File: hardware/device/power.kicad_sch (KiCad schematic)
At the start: 46 parts, among them IC3 SP3401-02UTG, J1 POT_CONN, J2 USB, U20 TPS62A02DRL, U21 TPS560200, U22 BQ24072RGT, U23 BQ21040DBV, U26 BQ25040, U31 FUSB302B01MPX, U32 LTC2942

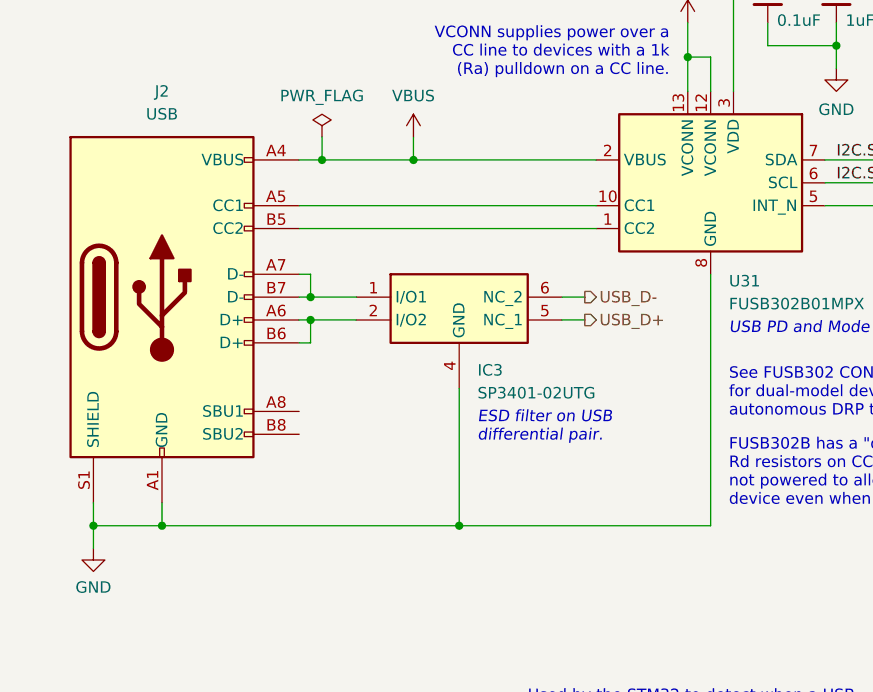
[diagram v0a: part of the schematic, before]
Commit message: feat: audio system routing
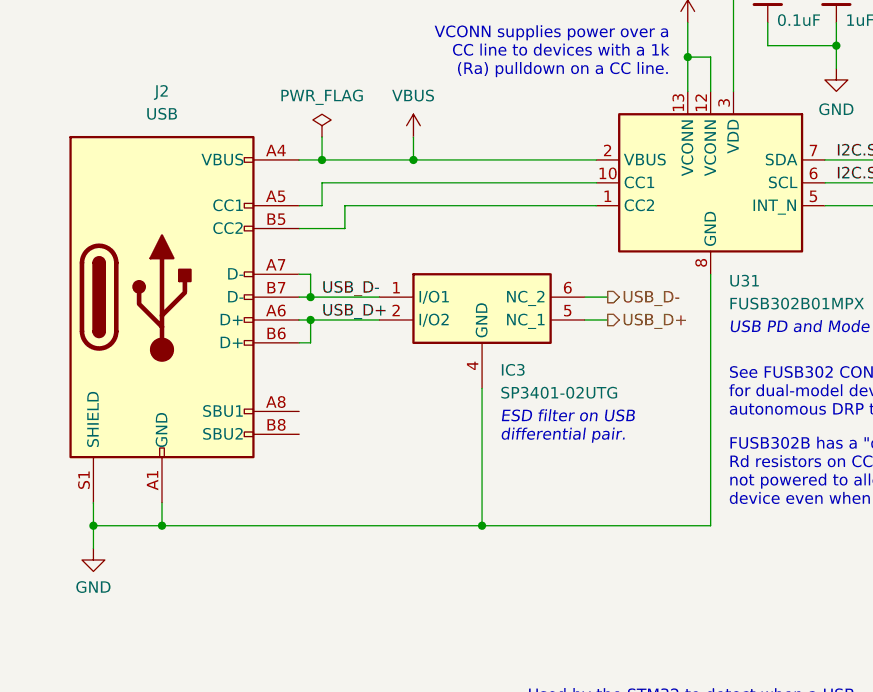
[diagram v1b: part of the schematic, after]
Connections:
- net USB_D+: now also IC3.2 (I/O2), J2.A6 (D+), J2.B6 (D+)
- net USB_D-: now also IC3.1 (I/O1), J2.A7 (D-), J2.B7 (D-)
- net at J2.B5 (CC2), U31.1 (CC2): now also U31.14 (CC2)
- net at J2.A5 (CC1), U31.10 (CC1): now also U31.11 (CC1); no longer U31.14 (CC2)
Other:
- moved on the sheet: IC3
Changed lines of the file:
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@@
 	(text "ESD filter on USB\ndifferential pair."
 		(exclude_from_sim no)
-		(at 64.262 76.2 0)
+		(at 66.802 76.2 0)
 		(effects
 			(font
@@
 	)
 	(junction
-		(at 62.23 88.9)
-		(diameter 0)
-		(color 0 0 0 0)
-	)
-	(junction
 		(at 76.2 153.67)
 		(diameter 0)
@@
 	)
 	(junction
+		(at 64.77 88.9)
+		(diameter 0)
+		(color 0 0 0 0)
+	)
+	(junction
 		(at 57.15 48.26)
 		(diameter 0)
@@
 	(wire
 		(pts
-			(xy 62.23 73.66) (xy 62.23 88.9)
+			(xy 64.77 73.66) (xy 64.77 88.9)
 		)
 		(stroke
@@
 	(wire
 		(pts
-			(xy 29.21 88.9) (xy 62.23 88.9)
+			(xy 29.21 88.9) (xy 64.77 88.9)
 		)
 		(stroke
@@
 		)
 	)
+	(wire
+		(pts
+			(xy 64.77 88.9) (xy 90.17 88.9)
+		)
+		(stroke
+			(width 0)
+			(type default)
+		)
+	)
 	(bus
 		(pts
@@
 	(wire
 		(pts
+			(xy 46.99 50.8) (xy 46.99 53.34)
+		)
+		(stroke
+			(width 0)
+			(type default)
+		)
+	)
+	(wire
+		(pts
 			(xy 132.08 158.75) (xy 130.81 158.75)
 		)
@@
 	(wire
 		(pts
-			(xy 73.66 63.5) (xy 76.2 63.5)
+			(xy 76.2 63.5) (xy 78.74 63.5)
 		)
 		(stroke
@@
 	(wire
 		(pts
-			(xy 62.23 88.9) (xy 90.17 88.9)
-		)
-		(stroke
-			(width 0)
-			(type default)
-		)
-	)
-	(wire
-		(pts
 			(xy 101.6 153.67) (xy 101.6 157.48)
 		)
@@
 	(wire
 		(pts
-			(xy 279.4 147.32) (xy 279.4 148.59)
+			(xy 49.53 53.34) (xy 77.47 53.34)
 		)
 		(stroke
@@
 	(wire
 		(pts
-			(xy 90.17 172.72) (xy 90.17 175.26)
+			(xy 279.4 147.32) (xy 279.4 148.59)
 		)
 		(stroke
@@
 	(wire
 		(pts
-			(xy 132.08 166.37) (xy 132.08 158.75)
+			(xy 90.17 172.72) (xy 90.17 175.26)
 		)
 		(stroke
@@
 	(wire
 		(pts
-			(xy 107.95 167.64) (xy 107.95 179.07)
+			(xy 132.08 166.37) (xy 132.08 158.75)
 		)
 		(stroke
@@
 	(wire
 		(pts
-			(xy 246.38 137.16) (xy 248.92 137.16)
+			(xy 107.95 167.64) (xy 107.95 179.07)
 		)
 		(stroke
@@
 	(wire
 		(pts
-			(xy 279.4 140.97) (xy 279.4 142.24)
+			(xy 246.38 137.16) (xy 248.92 137.16)
 		)
 		(stroke
@@
 	(wire
 		(pts
-			(xy 264.16 148.59) (xy 279.4 148.59)
+			(xy 279.4 140.97) (xy 279.4 142.24)
 		)
 		(stroke
@@
 	(wire
 		(pts
-			(xy 44.45 55.88) (xy 77.47 55.88)
+			(xy 264.16 148.59) (xy 279.4 148.59)
 		)
 		(stroke
@@
 	(wire
 		(pts
+			(xy 77.47 50.8) (xy 46.99 50.8)
+		)
+		(stroke
+			(width 0)
+			(type default)
+		)
+	)
+	(wire
+		(pts
 			(xy 271.78 88.9) (xy 271.78 86.36)
 		)
@@
 	(wire
 		(pts
+			(xy 44.45 55.88) (xy 49.53 55.88)
+		)
+		(stroke
+			(width 0)
+			(type default)
+		)
+	)
+	(wire
+		(pts
 			(xy 237.49 68.58) (xy 220.98 68.58)
 		)
@@
 	(wire
 		(pts
-			(xy 73.66 66.04) (xy 76.2 66.04)
+			(xy 76.2 66.04) (xy 78.74 66.04)
 		)
 		(stroke
@@
 	(wire
 		(pts
+			(xy 49.53 55.88) (xy 49.53 53.34)
+		)
+		(stroke
+			(width 0)
+			(type default)
+		)
+	)
+	(wire
+		(pts
 			(xy 271.78 68.58) (xy 271.78 71.12)
 		)
@@
 	(wire
 		(pts
-			(xy 50.8 63.5) (xy 45.72 63.5)
+			(xy 53.34 63.5) (xy 45.72 63.5)
 		)
 		(stroke
@@
 	(wire
 		(pts
-			(xy 44.45 53.34) (xy 77.47 53.34)
-		)
-		(stroke
-			(width 0)
-			(type default)
-		)
-	)
-	(wire
-		(pts
 			(xy 27.94 156.21) (xy 29.21 156.21)
 		)
@@
 	(wire
 		(pts
+			(xy 46.99 53.34) (xy 44.45 53.34)
+		)
+		(stroke
+			(width 0)
+			(type default)
+		)
+	)
+	(wire
+		(pts
 			(xy 57.15 153.67) (xy 67.31 153.67)
 		)
@@
 	(wire
 		(pts
-			(xy 50.8 66.04) (xy 45.72 66.04)
+			(xy 53.34 66.04) (xy 45.72 66.04)
 		)
 		(stroke
@@
 		)
 	)
+	(label "USB_D-"
+		(at 46.99 63.5 0)
+		(effects
+			(font
+				(size 1.27 1.27)
+			)
+			(justify left bottom)
+		)
+	)
 	(label "I2C.SDA"
 		(at 104.14 48.26 0)
@@
 		)
 	)
+	(label "USB_D+"
+		(at 46.99 66.04 0)
+		(effects
+			(font
+				(size 1.27 1.27)
+			)
+			(justify left bottom)
+		)
+	)
 	(label "I2C.SDA"
 		(at 236.22 68.58 180)
@@
 	(hierarchical_label "USB_D+"
 		(shape output)
-		(at 76.2 66.04 0)
+		(at 78.74 66.04 0)
 		(effects
 			(font
@@
 	(hierarchical_label "USB_D-"
 		(shape output)
-		(at 76.2 63.5 0)
+		(at 78.74 63.5 0)
 		(effects
 			(font
@@
 	)
 	(symbol
-		(lib_name "FUSB302B01MPX_1")
 		(lib_id "Interface_USB:FUSB302B01MPX")
 		(at 90.17 50.8 0)
@@
 	(symbol
 		(lib_id "pocket_synth:SP3401-02UTG")
-		(at 62.23 64.77 0)
+		(at 64.77 64.77 0)
 		(unit 1)
 		(exclude_from_sim no)
@@
 		(dnp no)
 		(property "Reference" "IC3"
-			(at 64.262 71.628 0)
+			(at 66.802 71.628 0)
 			(effects
 				(font
@@
 		)
 		(property "Value" "SP3401-02UTG"
-			(at 64.262 74.168 0)
+			(at 66.802 74.168 0)
 			(effects
 				(font
@@
 		)
 		(property "Footprint" "pocket_synth:SP340102UTG"
-			(at 88.9 159.69 0)
+			(at 91.44 159.69 0)
 			(effects
 				(font
@@
 		)
 		(property "Datasheet" "https://m.littelfuse.com/~/media/electronics/datasheets/tvs_diode_arrays/littelfuse_tvs_diode_array_sp3401_datasheet.pdf.pdf"
-			(at 88.9 259.69 0)
+			(at 91.44 259.69 0)
 			(effects
 				(font
@@
 		)
 		(property "Description" "ESD Suppressors / TVS Diodes 28KV 0.6pF 3.3V 10A uDFN-6 TVS Array"
-			(at 62.23 64.77 0)
+			(at 64.77 64.77 0)
 			(effects
 				(font
@@
 		)
 		(property "Height" "0.55"
-			(at 88.9 459.69 0)
+			(at 91.44 459.69 0)
 			(effects
 				(font
@@
 		)
 		(property "Mouser Part Number" "576-SP3401-02UTG"
-			(at 88.9 559.69 0)
+			(at 91.44 559.69 0)
 			(effects
 				(font
@@
 		)
 		(property "Mouser Price/Stock" "https://www.mouser.co.uk/ProductDetail/Littelfuse/SP3401-02UTG?qs=T3oQrply3y%2FjRDLmSQJ5ww%3D%3D"
-			(at 88.9 659.69 0)
+			(at 91.44 659.69 0)
 			(effects
 				(font
@@
 		)
 		(property "Manufacturer_Name" "LITTELFUSE"
-			(at 88.9 759.69 0)
+			(at 91.44 759.69 0)
 			(effects
 				(font
@@
 		)
 		(property "Manufacturer_Part_Number" "SP3401-02UTG"
-			(at 88.9 859.69 0)
+			(at 91.44 859.69 0)
 			(effects
 				(font
@@
 		)
 		(property "JLC" "C3702190"
-			(at 62.23 64.77 0)
+			(at 64.77 64.77 0)
 			(effects
 				(font
